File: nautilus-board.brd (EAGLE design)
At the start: 50.8 x 22.9 mm, 35 parts, among them Q3 DMG2305, SW1 KMR2, U1 2MB Flash, U2 AP2112(3.3V), U3 MCP73831T-2ACI/OT, X1 JSTPH, X2 4u20329

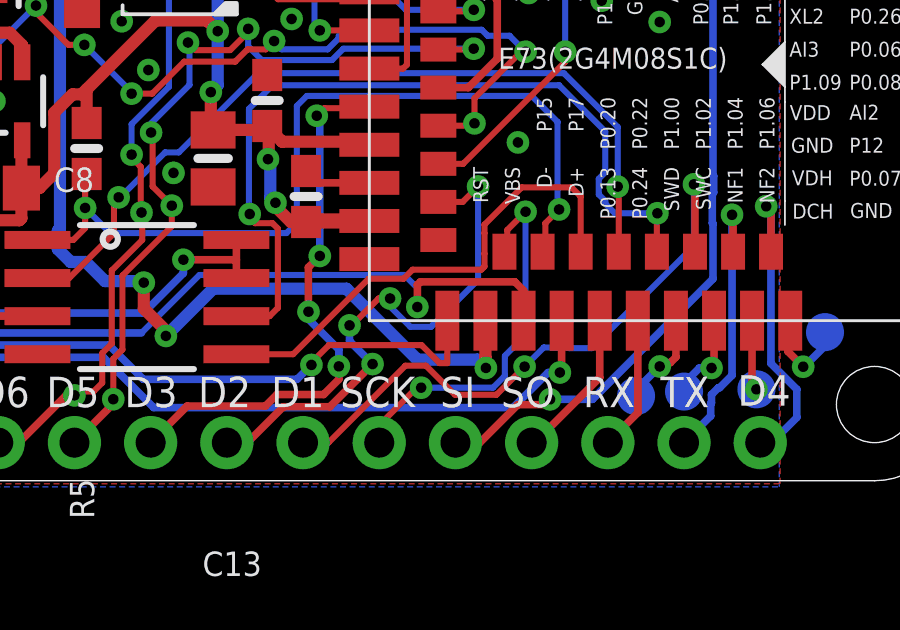
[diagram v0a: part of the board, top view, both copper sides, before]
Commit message: Adjusted traces
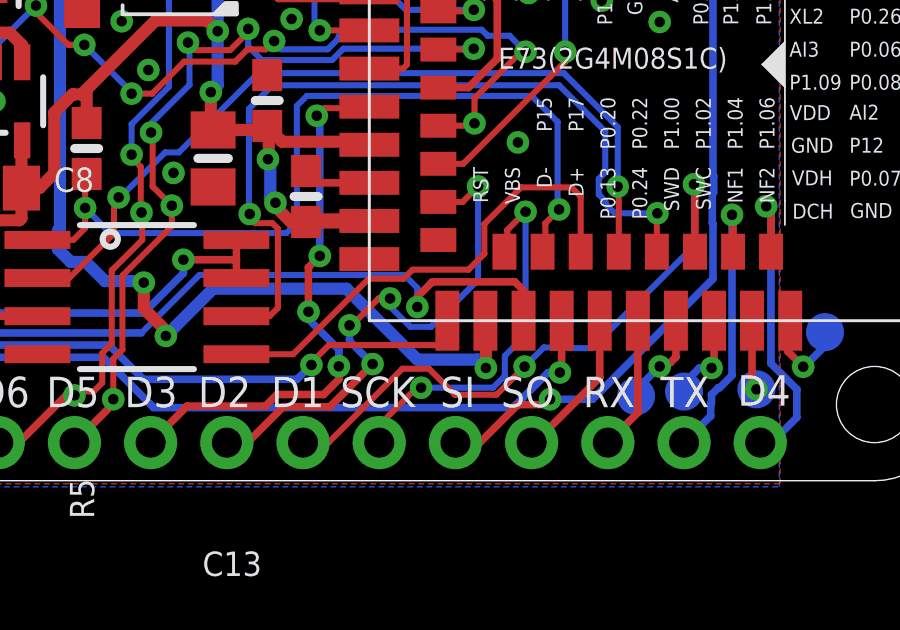
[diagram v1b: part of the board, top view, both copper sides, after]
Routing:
- net RESET: track 33.8 -> 32.9 mm
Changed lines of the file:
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@@
 <drawing>
 <settings>
-<setting alwaysvectorfont="yes"/>
+<setting alwaysvectorfont="no"/>
 <setting verticaltext="up"/>
 </settings>
@@
 <wire x1="14.4018" y1="8.7989" x2="14.417" y2="8.7837" width="0.4064" layer="1"/>
 <via x="20.2184" y="20.1422" extent="1-16" drill="0.35"/>
-<wire x1="35.2898" y1="5.334" x2="35.2898" y2="4.0986" width="0.4064" layer="1"/>
-<wire x1="35.2898" y1="4.0986" x2="35.2806" y2="4.0894" width="0.4064" layer="1"/>
-<wire x1="35.306" y1="4.064" x2="35.306" y2="3.7592" width="0.4064" layer="1"/>
-<wire x1="35.306" y1="4.064" x2="35.2806" y2="4.0894" width="0.4064" layer="1"/>
+<wire x1="35.2898" y1="5.334" x2="35.306" y2="5.3178" width="0.4064" layer="1"/>
+<wire x1="35.306" y1="5.3178" x2="35.306" y2="3.7592" width="0.4064" layer="1"/>
 <via x="35.306" y="3.7592" extent="1-16" drill="0.35"/>
 <wire x1="20.2184" y1="20.1422" x2="20.32" y2="20.0406" width="0.4064" layer="1"/>
@@
 <wire x1="22.7428125" y1="4.5212" x2="17.2851" y2="4.5212" width="0.254" layer="16"/>
 <wire x1="17.2851" y1="4.5212" x2="16.8148" y2="4.0509" width="0.254" layer="16"/>
-<wire x1="34.0198" y1="5.334" x2="34.0198" y2="3.9208" width="0.2032" layer="1"/>
-<wire x1="34.0198" y1="3.9208" x2="33.7606875" y2="3.9208" width="0.2032" layer="1"/>
-<wire x1="33.7606875" y1="3.9208" x2="33.1602875" y2="4.5212" width="0.2032" layer="1"/>
-<wire x1="33.1602875" y1="4.5212" x2="30.0736" y2="4.5212" width="0.2032" layer="1"/>
+<wire x1="34.0198" y1="5.334" x2="34.0198" y2="4.5212" width="0.2032" layer="1"/>
+<wire x1="34.0198" y1="4.5212" x2="30.0736" y2="4.5212" width="0.2032" layer="1"/>
 <wire x1="30.0736" y1="4.5212" x2="29.4894" y2="3.937" width="0.2032" layer="1"/>
 <wire x1="29.4894" y1="3.8608" x2="29.4894" y2="3.937" width="0.2032" layer="1"/>
@@
 <contactref element="U1" pad="5"/>
 <wire x1="28.87981875" y1="4.2164" x2="26.9878" y2="4.2164" width="0.2032" layer="1"/>
-<wire x1="35.1536" y1="7.0358" x2="32.86218125" y2="7.0358" width="0.2032" layer="1"/>
 <wire x1="32.86218125" y1="7.0358" x2="32.560090625" y2="6.733709375" width="0.2032" layer="1"/>
 <wire x1="38.4648" y1="7.634" x2="38.4648" y2="9.4742" width="0.2032" layer="1"/>
-<wire x1="35.258" y1="7.1402" x2="35.1536" y2="7.0358" width="0.2032" layer="1"/>
-<wire x1="36.4998" y1="9.779" x2="35.258" y2="8.5372" width="0.2032" layer="1"/>
-<wire x1="35.258" y1="8.5372" x2="35.258" y2="8.255" width="0.2032" layer="1"/>
-<wire x1="35.258" y1="8.255" x2="35.258" y2="7.5692" width="0.2032" layer="1"/>
-<wire x1="35.258" y1="7.5692" x2="35.258" y2="7.1402" width="0.2032" layer="1"/>
 <wire x1="32.560090625" y1="6.733709375" x2="31.39710625" y2="6.733709375" width="0.2032" layer="1"/>
 <wire x1="31.39710625" y1="6.733709375" x2="28.87981875" y2="4.2164" width="0.2032" layer="1"/>
 <wire x1="38.4648" y1="9.4742" x2="38.16" y2="9.779" width="0.2032" layer="1"/>
-<wire x1="38.16" y1="9.779" x2="36.4998" y2="9.779" width="0.2032" layer="1"/>
+<wire x1="38.16" y1="9.779" x2="36.4744" y2="9.779" width="0.2032" layer="1"/>
+<wire x1="35.2566" y1="7.5678" x2="34.7246" y2="7.0358" width="0.2032" layer="1"/>
+<wire x1="34.7246" y1="7.0358" x2="32.86218125" y2="7.0358" width="0.2032" layer="1"/>
+<wire x1="35.2566" y1="8.5612" x2="35.2566" y2="7.5678" width="0.2032" layer="1"/>
+<wire x1="36.4744" y1="9.779" x2="35.2566" y2="8.5612" width="0.2032" layer="1"/>
 </signal>
 <signal name="SPI_FLASH_CS_PIN">
@@
 <wire x1="7.7216" y1="7.8486" x2="7.874" y2="8.001" width="0.254" layer="16"/>
 <via x="33.02" y="5.7912" extent="1-16" drill="0.35"/>
-<wire x1="36.2712" y1="6.6294" x2="33.1216" y2="6.6294" width="0.254" layer="1"/>
-<wire x1="33.1216" y1="6.6294" x2="33.02" y2="6.5278" width="0.254" layer="1"/>
-<wire x1="33.02" y1="6.5278" x2="33.02" y2="5.7912" width="0.254" layer="1"/>
+<wire x1="36.2712" y1="6.6294" x2="33.528" y2="6.6294" width="0.254" layer="1"/>
 <wire x1="36.5598" y1="5.334" x2="36.5598" y2="6.3408" width="0.254" layer="1"/>
-<wire x1="36.5598" y1="6.3408" x2="36.2712" y2="6.6294" width="0.254" layer="1"/>
+<wire x1="36.2712" y1="6.6294" x2="36.5598" y2="6.3408" width="0.254" layer="1"/>
 <wire x1="23.8252" y1="4.9276" x2="25.7556" y2="6.858" width="0.2032" layer="16"/>
 <wire x1="25.7556" y1="6.858" x2="32.5882" y2="6.858" width="0.2032" layer="16"/>
@@
 <wire x1="12.4206" y1="8.001" x2="15.494" y2="4.9276" width="0.254" layer="16"/>
 <wire x1="15.494" y1="4.9276" x2="23.8252" y2="4.9276" width="0.254" layer="16"/>
+<wire x1="33.528" y1="6.6294" x2="33.512" y2="6.6134" width="0.254" layer="1"/>
+<wire x1="33.512" y1="6.6134" x2="33.50406875" y2="6.6134" width="0.254" layer="1"/>
+<wire x1="33.50406875" y1="6.6134" x2="33.02" y2="6.12933125" width="0.254" layer="1"/>
+<wire x1="33.02" y1="6.12933125" x2="33.02" y2="5.7912" width="0.254" layer="1"/>
 </signal>
 <signal name="D+1">
@@
 <via x="42.2402" y="9.8806" extent="1-16" drill="0.35"/>
 <via x="36.5948" y="3.8034" extent="1-16" drill="0.35"/>
-<wire x1="32.62275" y1="3.8354" x2="30.05735" y2="1.27" width="0.2032" layer="1"/>
+<wire x1="32.52115" y1="3.7338" x2="30.05735" y2="1.27" width="0.2032" layer="1"/>
 <wire x1="29.21" y1="1.27" x2="30.05735" y2="1.27" width="0.2032" layer="1"/>
-<wire x1="32.62275" y1="3.8354" x2="33.30726875" y2="3.8354" width="0.2032" layer="1"/>
+<wire x1="32.52115" y1="3.7338" x2="33.40886875" y2="3.7338" width="0.2032" layer="1"/>
 <wire x1="35.65653125" y1="2.86513125" x2="36.5948" y2="3.8034" width="0.2032" layer="1"/>
 <wire x1="34.2775375" y1="2.86513125" x2="35.65653125" y2="2.86513125" width="0.2032" layer="1"/>
-<wire x1="33.30726875" y1="3.8354" x2="34.2775375" y2="2.86513125" width="0.2032" layer="1"/>
+<wire x1="33.40886875" y1="3.7338" x2="34.2775375" y2="2.86513125" width="0.2032" layer="1"/>
 <wire x1="42.2402" y1="9.8806" x2="42.2402" y2="7.8232" width="0.2032" layer="16"/>
 <wire x1="42.2402" y1="7.8232" x2="38.8366" y2="4.4196" width="0.2032" layer="16"/>
